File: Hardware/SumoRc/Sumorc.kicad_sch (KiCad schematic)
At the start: 9 parts, among them J1 Screw_Terminal_01x08, J2 Screw_Terminal_01x08, SW1 SW_SPDT, U1 ESP32_DevKit_V1_DOIT, U2 LF15_TO220

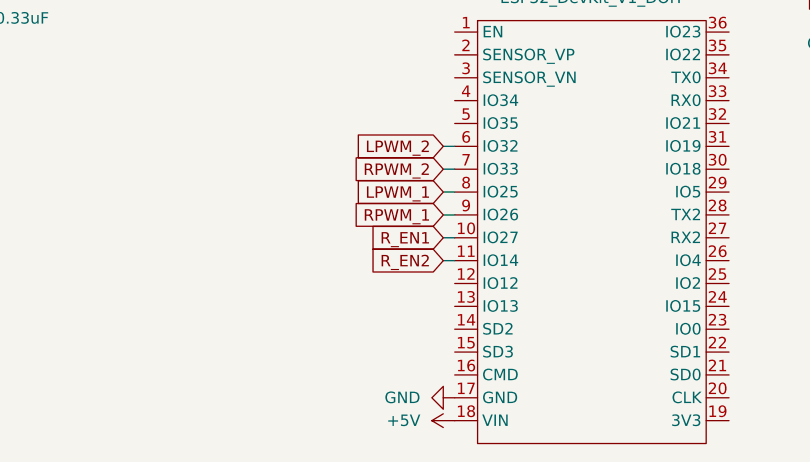
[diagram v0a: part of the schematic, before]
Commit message: actualizacion
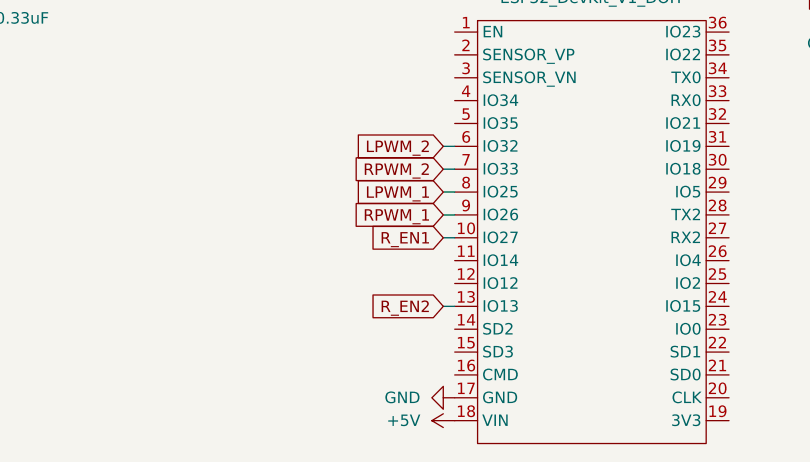
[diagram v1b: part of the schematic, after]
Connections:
- net L_EN2: now also U1.13 (IO13); no longer U1.11 (IO14)
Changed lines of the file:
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@@
-	(wire
-		(pts
-			(xy 113.03 80.01) (xy 114.3 80.01)
-		)
-		(stroke
-			(width 0)
-			(type default)
-		)
-	)
 	(wire
 		(pts
@@
 		(pts
 			(xy 195.58 48.26) (xy 194.31 48.26)
+		)
+		(stroke
+			(width 0)
+			(type default)
+		)
+	)
+	(wire
+		(pts
+			(xy 113.03 85.09) (xy 114.3 85.09)
 		)
 		(stroke
@@
 	(global_label "R_EN2"
 		(shape input)
-		(at 113.03 80.01 180)
-		(fields_autoplaced yes)
-		(effects
-			(font
-				(size 1.27 1.27)
-			)
-			(justify right)
-		)
-		(property "Intersheetrefs" "${INTERSHEET_REFS}"
-			(at 104.1182 80.01 0)
-			(effects
-				(font
+		(at 113.03 85.09 180)
+		(fields_autoplaced yes)
+		(effects
+			(font
+				(size 1.27 1.27)
+			)
+			(justify right)
+		)
+		(property "Intersheetrefs" "${INTERSHEET_REFS}"
+			(at 104.1182 85.09 0)
+			(effects
+				(font

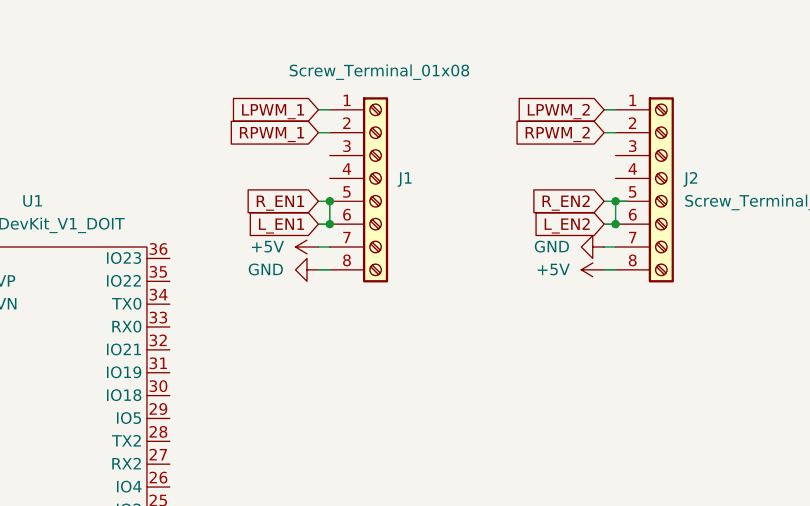
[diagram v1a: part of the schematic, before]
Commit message: actualizacion
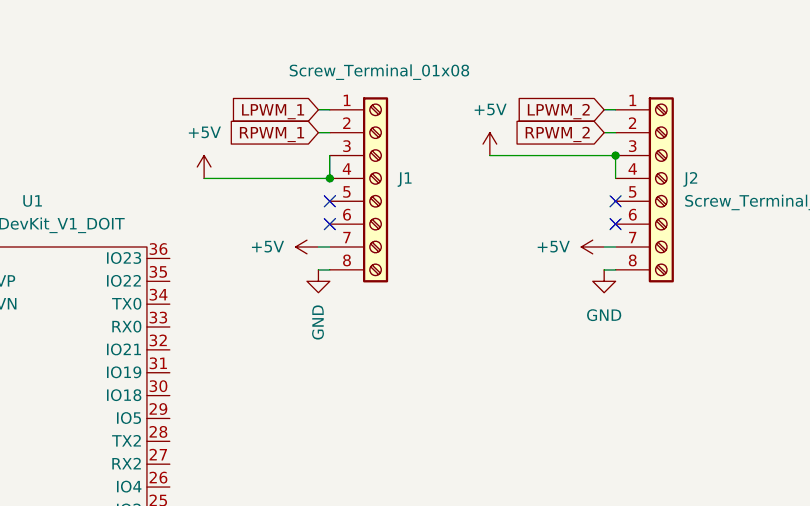
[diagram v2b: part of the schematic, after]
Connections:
- net +5V: now also J1.3 (Pin_3), J1.4 (Pin_4), J2.3 (Pin_3), J2.4 (Pin_4), J2.7 (Pin_7); no longer J2.8 (Pin_8)
- net GND: now also J2.8 (Pin_8); no longer J2.7 (Pin_7)
- removed net L_EN1: J1.5 (Pin_5), J1.6 (Pin_6), U1.10 (IO27)
- removed net L_EN2: J2.5 (Pin_5), J2.6 (Pin_6), U1.13 (IO13)
- new net R_EN1: U1.10 (IO27)
- new net R_EN2: U1.13 (IO13)
- no-connect marks 0 -> 4
